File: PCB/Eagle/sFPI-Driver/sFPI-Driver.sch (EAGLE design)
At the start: 34 parts, among them IC1 ATMEGA168-PU, T1 POTMILRV8-SPR, T2 POTMILRV8-SPR, T3 POTMILRV8-SPR, T4 POTMILRV8-SPR, U1 LT1006CN8PBF, U2 LT1006CN8PBF, U3 LT1006CN8PBF, U4 LT1006CN8PBF, U5 LT1006CN8PBF, U6 LT1006CN8PBF

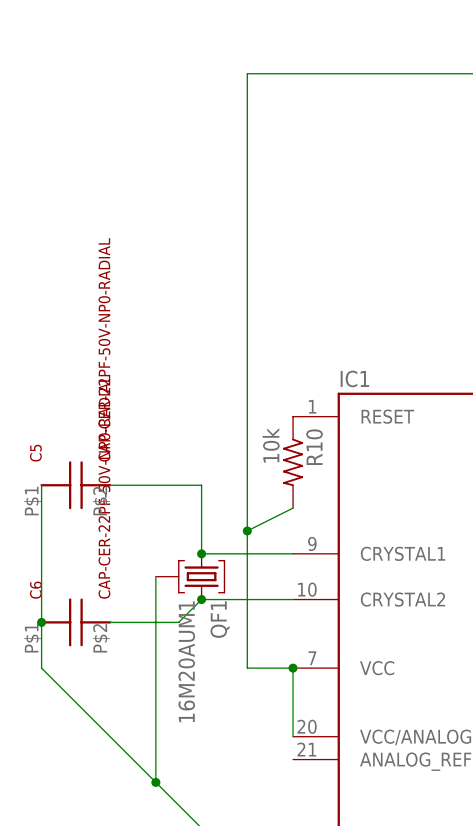
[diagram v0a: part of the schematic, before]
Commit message: ReEdited Paper with final changes
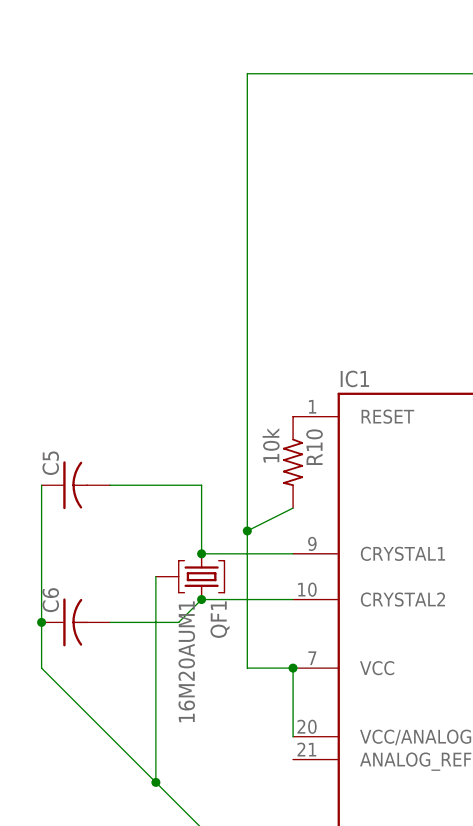
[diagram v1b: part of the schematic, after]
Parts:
- C5, C6: value CAP-CER-22PF-50V-NP0-RADIAL -> (none); device sFPI:CAP-CER-22PF-50V-NP0-RADIAL -> rcl:C-US025-024X044
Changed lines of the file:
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@@
 <part name="C8" library="sFPI" deviceset="CAP-CER-22PF-50V-NP0-RADIAL" device=""/>
 <part name="C9" library="sFPI" deviceset="CAP-CER-22PF-50V-NP0-RADIAL" device=""/>
-<part name="C5" library="sFPI" deviceset="CAP-CER-22PF-50V-NP0-RADIAL" device=""/>
-<part name="C6" library="sFPI" deviceset="CAP-CER-22PF-50V-NP0-RADIAL" device=""/>
 <part name="R1" library="rcl" deviceset="R-US_" device="0207/10" value="10k"/>
 <part name="R2" library="rcl" deviceset="R-US_" device="0207/10" value="10k"/>
@@
 <part name="T2" library="sFPI" deviceset="POTMILRV8" device="-SPR"/>
 <part name="T3" library="sFPI" deviceset="POTMILRV8" device="-SPR"/>
+<part name="C5" library="rcl" deviceset="C-US" device="025-024X044"/>
+<part name="C6" library="rcl" deviceset="C-US" device="025-024X044"/>
 </parts>
 <sheets>
@@
 <instance part="C8" gate="G$1" x="213.36" y="91.44"/>
 <instance part="C9" gate="G$1" x="299.72" y="91.44"/>
-<instance part="C5" gate="G$1" x="-30.48" y="81.28" rot="R90"/>
-<instance part="C6" gate="G$1" x="-30.48" y="66.04" rot="R90"/>
 <instance part="R1" gate="G$1" x="132.08" y="76.2"/>
 <instance part="R2" gate="G$1" x="157.48" y="99.06"/>
@@
 <instance part="T2" gate="G$1" x="198.12" y="83.82"/>
 <instance part="T3" gate="G$1" x="119.38" y="76.2"/>
+<instance part="C5" gate="G$1" x="-33.02" y="81.28" rot="R90"/>
+<instance part="C6" gate="G$1" x="-33.02" y="66.04" rot="R90"/>
 </instances>
 <busses>
